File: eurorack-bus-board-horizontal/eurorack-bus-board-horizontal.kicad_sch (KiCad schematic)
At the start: 13 parts, among them J1 Power IN/THRU, J10 Conn_02x08_Eurorack, J2 Conn_02x08_Eurorack, J3 Conn_02x08_Eurorack, J5 Conn_02x08_Eurorack, J6 Conn_02x08_Eurorack, J7 Conn_02x08_Eurorack, J8 Conn_02x08_Eurorack, J9 Conn_02x08_Eurorack

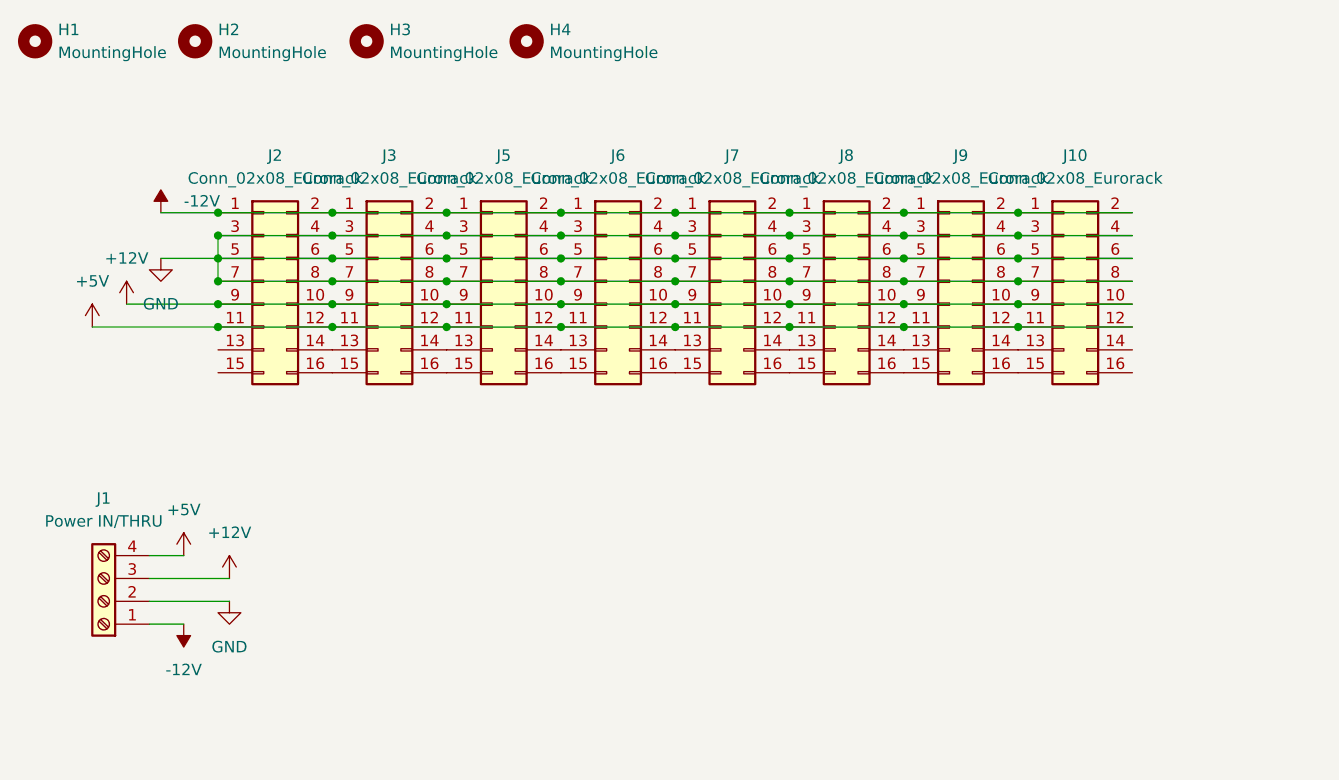
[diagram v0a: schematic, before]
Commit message: add additional files
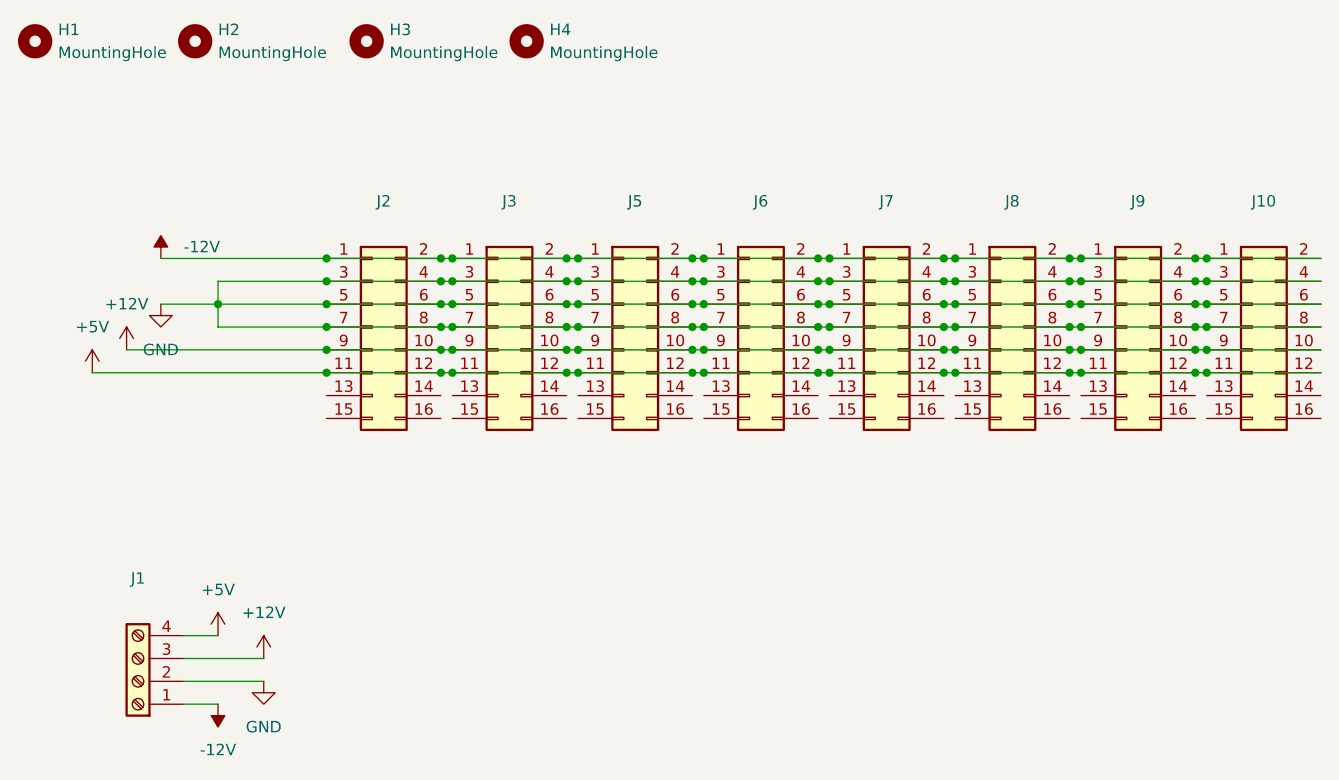
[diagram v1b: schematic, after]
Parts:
- J1: value Power IN/THRU -> (none)
- J10, J2, J3, J5, J6, J7, J8, J9: value Conn_02x08_Eurorack -> (none); footprint Connector_IDC:IDC-Header_2x08_P2.54mm_Horizontal -> (none)
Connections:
- net at J8.13 (Pin_13): no longer J7.14 (Pin_14)
- net at J8.14 (Pin_14): no longer J9.13 (Pin_13)
- net at J8.15 (Pin_15): no longer J7.16 (Pin_16)
- net at J8.16 (Pin_16): no longer J9.15 (Pin_15)
- net at J2.14 (Pin_14): no longer J3.13 (Pin_13)
- net at J2.16 (Pin_16): no longer J3.15 (Pin_15)
- net at J5.13 (Pin_13): no longer J3.14 (Pin_14)
- net at J5.14 (Pin_14): no longer J6.13 (Pin_13)
- net at J5.15 (Pin_15): no longer J3.16 (Pin_16)
- net at J5.16 (Pin_16): no longer J6.15 (Pin_15)
- net at J6.14 (Pin_14): no longer J7.13 (Pin_13)
- net at J6.16 (Pin_16): no longer J7.15 (Pin_15)
- net at J10.13 (Pin_13): no longer J9.14 (Pin_14)
- net at J10.15 (Pin_15): no longer J9.16 (Pin_16)
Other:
- moved on the sheet: J1, J10, J2, J3, J5, J6, J7, J8, J9
